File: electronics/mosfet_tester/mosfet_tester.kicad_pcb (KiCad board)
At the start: 2 copper layers, 25 parts, among them J101 BARREL_JACK, J102 CONN_01X06, J103 Screw_Terminal_1x01, J104 Screw_Terminal_1x01, J201 TEST_1P, J202 TEST_1P, J203 TEST_1P, J205 TEST_1P, J206 TEST_1P, J207 TEST_1P, Q201 Q_NMOS_GSD, U101 LM7805CT, U201 LM358

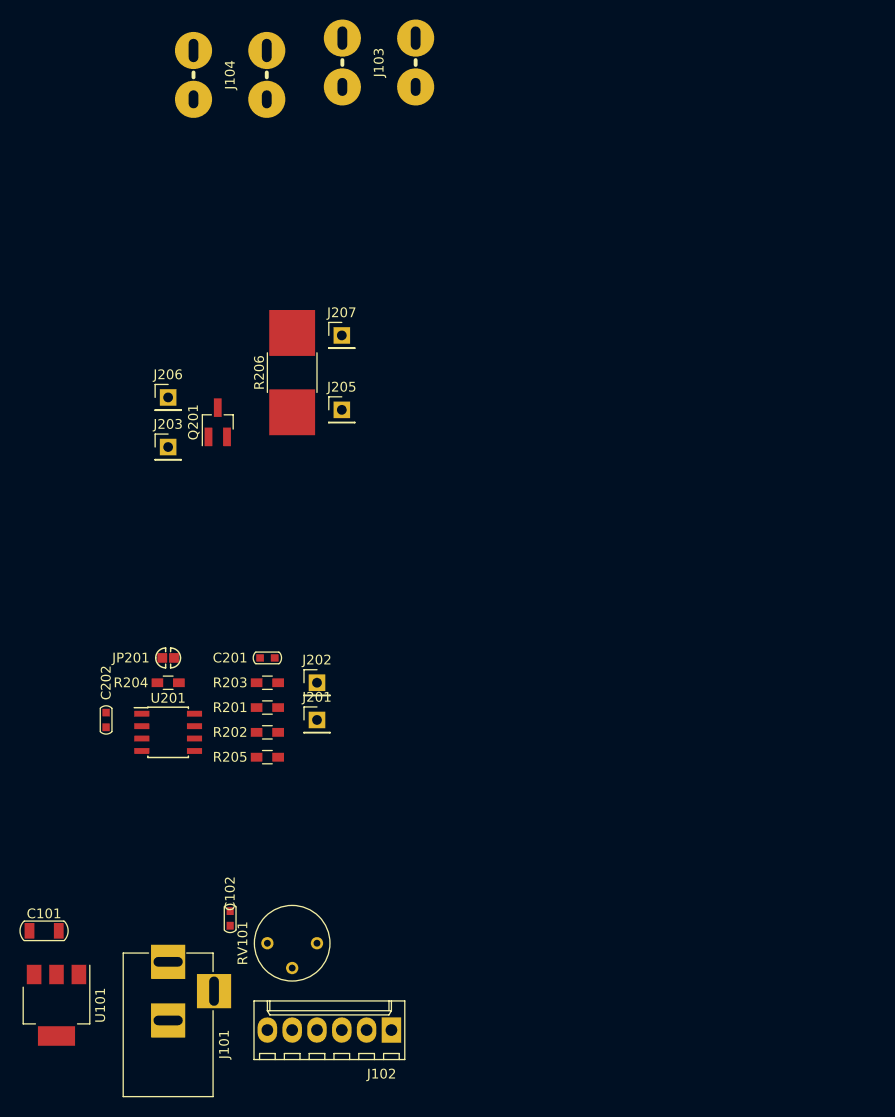
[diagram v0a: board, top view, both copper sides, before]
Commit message: Rework entire board, still in progress
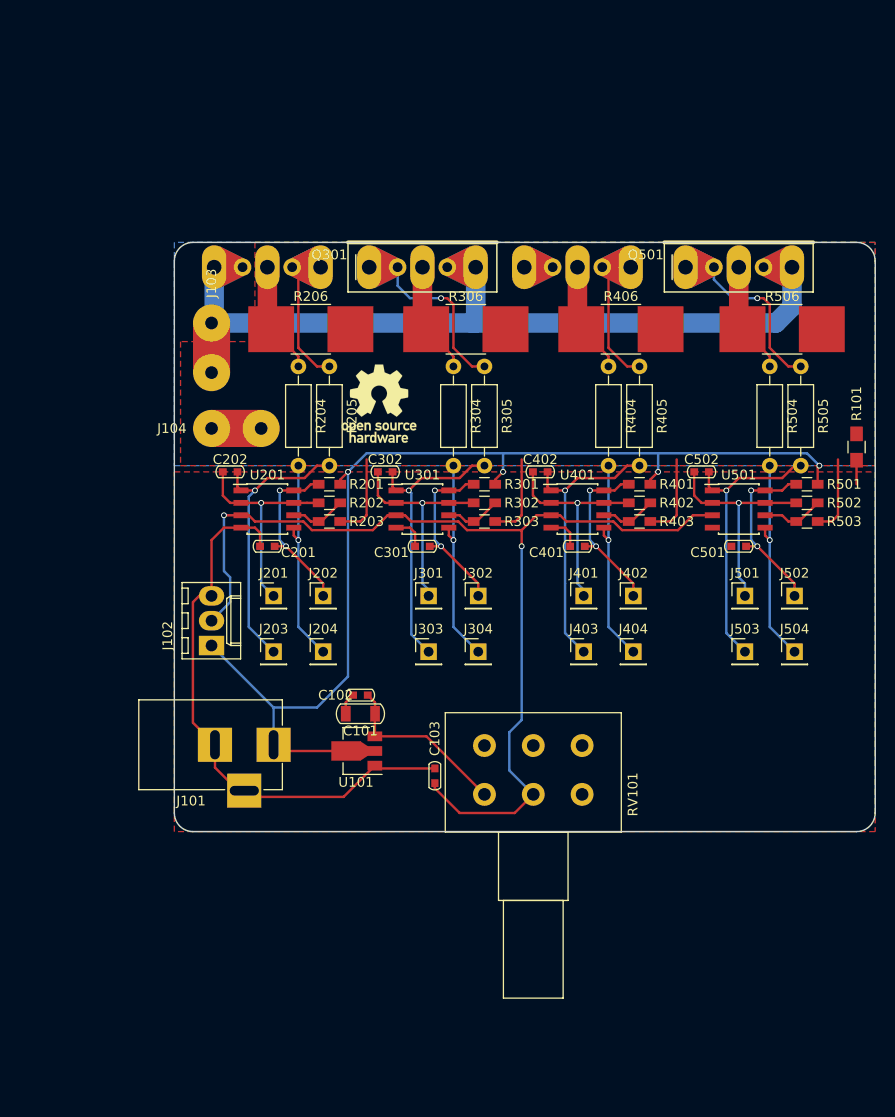
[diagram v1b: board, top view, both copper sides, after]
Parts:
- removed J206, J207: TEST_1P, Pin_Headers:Pin_Header_Straight_1x01_Pitch2.54mm
- removed JP201: Jumper_NC_Small, SolderJumpers:SJ_1_NO
- added C102: 0.1u, Capacitors_SMD_Round:C_0603, F.Cu at (135.3, 123.2)
- added C301: 0.1, Capacitors_SMD_Round:C_0603, F.Cu at (141.6, 108.0)
- added C302: C, Capacitors_SMD_Round:C_0603, F.Cu at (137.8, 100.3)
- added C401: 0.1, Capacitors_SMD_Round:C_0603, F.Cu at (157.5, 108.0)
- added C402: C, Capacitors_SMD_Round:C_0603, F.Cu at (153.7, 100.3)
- added C501: 0.1, Capacitors_SMD_Round:C_0603, F.Cu at (174.0, 108.0)
- added C502: C, Capacitors_SMD_Round:C_0603, F.Cu at (170.2, 100.3)
- added J301: TEST_1P, Pin_Headers:Pin_Header_Straight_1x01_Pitch2.54mm, F.Cu at (142.2, 113.0)
- added J302: TEST_1P, Pin_Headers:Pin_Header_Straight_1x01_Pitch2.54mm, F.Cu at (147.3, 113.0)
- added J303: TEST_1P, Pin_Headers:Pin_Header_Straight_1x01_Pitch2.54mm, F.Cu at (142.2, 118.7)
- added J304: TEST_1P, Pin_Headers:Pin_Header_Straight_1x01_Pitch2.54mm, F.Cu at (147.3, 118.7)
- added J401: TEST_1P, Pin_Headers:Pin_Header_Straight_1x01_Pitch2.54mm, F.Cu at (158.1, 113.0)
- added J402: TEST_1P, Pin_Headers:Pin_Header_Straight_1x01_Pitch2.54mm, F.Cu at (163.2, 113.0)
- added J403: TEST_1P, Pin_Headers:Pin_Header_Straight_1x01_Pitch2.54mm, F.Cu at (158.1, 118.7)
- added J404: TEST_1P, Pin_Headers:Pin_Header_Straight_1x01_Pitch2.54mm, F.Cu at (163.2, 118.7)
- added J501: TEST_1P, Pin_Headers:Pin_Header_Straight_1x01_Pitch2.54mm, F.Cu at (174.6, 113.0)
- added J502: TEST_1P, Pin_Headers:Pin_Header_Straight_1x01_Pitch2.54mm, F.Cu at (179.7, 113.0)
- added J503: TEST_1P, Pin_Headers:Pin_Header_Straight_1x01_Pitch2.54mm, F.Cu at (174.6, 118.7)
- added J504: TEST_1P, Pin_Headers:Pin_Header_Straight_1x01_Pitch2.54mm, F.Cu at (179.7, 118.7)
- added P101: OSHW, Symbols:OSHW-Logo_7.5x8mm_SilkScreen, F.Cu at (137.2, 93.3)
- added Q301: Q_NMOS_GSD, TO_Combo_Packages:TO_220_247, F.Cu at (141.6, 79.4)
- added Q401: Q_NMOS_GSD, TO_Combo_Packages:TO_220_247, B.Cu at (157.5, 79.4)
- added Q501: Q_NMOS_GSD, TO_Combo_Packages:TO_220_247, F.Cu at (174.0, 79.4)
- added R101: 0R, Resistors_SMD:R_0805_HandSoldering, F.Cu at (186.1, 97.8)
- added R301: 100R, Resistors_SMD:R_0603_HandSoldering, F.Cu at (148.0, 101.6)
- added R302: R, Resistors_SMD:R_0603_HandSoldering, F.Cu at (148.0, 103.5)
- added R303: R, Resistors_SMD:R_0603_HandSoldering, F.Cu at (148.0, 105.4)
- added R304: R, Resistors_THT:R_Axial_DIN0207_L6.3mm_D2.5mm_P10.16mm_Horizontal, F.Cu at (144.8, 89.5)
- added R305: R, Resistors_THT:R_Axial_DIN0207_L6.3mm_D2.5mm_P10.16mm_Horizontal, F.Cu at (148.0, 89.5)
- added R306: R, Resistors_SMD:R_2816_HandSoldering, F.Cu at (146.1, 85.7)
- added R401: 100R, Resistors_SMD:R_0603_HandSoldering, F.Cu at (163.8, 101.6)
- added R402: R, Resistors_SMD:R_0603_HandSoldering, F.Cu at (163.8, 103.5)
- added R403: R, Resistors_SMD:R_0603_HandSoldering, F.Cu at (163.8, 105.4)
- added R404: R, Resistors_THT:R_Axial_DIN0207_L6.3mm_D2.5mm_P10.16mm_Horizontal, F.Cu at (160.7, 89.5)
- added R405: R, Resistors_THT:R_Axial_DIN0207_L6.3mm_D2.5mm_P10.16mm_Horizontal, F.Cu at (163.8, 89.5)
- added R406: R, Resistors_SMD:R_2816_HandSoldering, F.Cu at (161.9, 85.7)
- added R501: 100R, Resistors_SMD:R_0603_HandSoldering, F.Cu at (181.0, 101.6)
- added R502: R, Resistors_SMD:R_0603_HandSoldering, F.Cu at (181.0, 103.5)
- added R503: R, Resistors_SMD:R_0603_HandSoldering, F.Cu at (181.0, 105.4)
- added R504: R, Resistors_THT:R_Axial_DIN0207_L6.3mm_D2.5mm_P10.16mm_Horizontal, F.Cu at (177.2, 89.5)
- added R505: R, Resistors_THT:R_Axial_DIN0207_L6.3mm_D2.5mm_P10.16mm_Horizontal, F.Cu at (180.3, 89.5)
- added R506: R, Resistors_SMD:R_2816_HandSoldering, F.Cu at (178.4, 85.7)
- added U301: LM358, Housings_SOIC:SOIC-8_3.9x4.9mm_Pitch1.27mm, F.Cu at (141.6, 104.1)
- added U401: LM358, Housings_SOIC:SOIC-8_3.9x4.9mm_Pitch1.27mm, F.Cu at (157.5, 104.1)
- added U501: LM358, Housings_SOIC:SOIC-8_3.9x4.9mm_Pitch1.27mm, F.Cu at (174.0, 104.1)
- C101: value C -> 22u
- J102: value CONN_01X06 -> CONN_01X03; footprint Connectors_Molex:Molex_KK-6410-06_06x2.54mm_Straight -> Connectors_Molex:Molex_KK-6410-03_03x2.54mm_Straight
- J103, J104: footprint Screw_Connectors:4_Pin_Screw_Connector -> Screw_Connectors:2_Pin_Quick_Fit
- Q201: footprint TO_SOT_Packages_SMD:SOT-23_Handsoldering -> TO_Combo_Packages:TO_220_247; moved to B.Cu
- R204, R205: footprint Resistors_SMD:R_0603_HandSoldering -> Resistors_THT:R_Axial_DIN0207_L6.3mm_D2.5mm_P10.16mm_Horizontal
- RV101: footprint Potentiometers:Potentiometer_Trimmer_Bourns_3339P_Horizontal -> Potentiometers:Potentiometer_Alps_RK163_Double_Vertical
- U101: value LM7805CT -> MCP1703A-3302/MB; footprint TO_SOT_Packages_SMD:SOT-223-3Lead_TabPin2 -> TO_SOT_Packages_SMD:SOT89-3_Housing
- moved J102 43.5 mm to (120.0, 118.1), turned to 90 degrees
- moved U101 40.6 mm to (135.3, 128.9), turned to 180 degrees
- moved R205 40.5 mm to (132.1, 89.5), turned to 270 degrees
- moved C101 39.3 mm to (135.3, 125.1), turned to 180 degrees
- moved J104 36.2 mm to (122.6, 95.9), turned to 0 degrees
- moved R204 35.0 mm to (128.9, 89.5), turned to 270 degrees
- moved J103 33.9 mm to (120.0, 87.6), turned to 270 degrees
- moved C202 28.4 mm to (121.9, 100.3), turned to 180 degrees
- moved C103 25.5 mm to (142.9, 131.4)
- moved U201 25.0 mm to (125.7, 104.1)
- moved J204 24.8 mm to (131.4, 118.7)
- moved J101 24.7 mm to (126.4, 128.3), turned to 0 degrees
- moved R202 24.3 mm to (132.1, 103.5)
- moved R201 23.7 mm to (132.1, 101.6)
- moved J203 23.6 mm to (126.4, 118.7)
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- renumbered C102 to C103, J205 to J204
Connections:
- C103 pad 1: /slice/5V_REF -> /slice1/5V_REF
- C202 pad 1: Net-(C202-Pad1) -> /slice1/Vgs
- J102 pad 1: /slice/Vgs -> +12V
- J102 pad 2: (no net) -> /slice1/5V_REF
- J102 pad 3: (no net) -> GND
- J103 pad 1: GND -> /slice1/VIN+
- J104 pad 1: /slice/VIN+ -> /slice1/VIN-
- J203 pad 1: /slice/Vgs -> /slice1/Vgs
- J204 pad 1: Net-(J205-Pad1) -> Net-(J204-Pad1)
- Q201 pad 1: /slice/Vgs -> Net-(Q201-Pad1)
- Q201 pad 2: Net-(J205-Pad1) -> Net-(Q201-Pad2)
- Q201 pad 3: /slice/VIN+ -> /slice1/VIN+
- R203 pad 1: Net-(JP201-Pad1) -> /slice1/VIN-
- R204 pad 1: /slice/Vgs -> Net-(Q201-Pad2)
- R204 pad 2: Net-(C202-Pad1) -> Net-(J204-Pad1)
- R205 pad 1: Net-(J205-Pad1) -> Net-(Q201-Pad1)
- R205 pad 2: Net-(R205-Pad2) -> /slice1/Vgs
- R206 pad 1: Net-(J205-Pad1) -> Net-(Q201-Pad2)
- R206 pad 2: GND -> /slice1/VIN-
- RV101 pad 2: /slice/5V_REF -> /slice1/5V_REF
- U101 pad 1: +12V -> GND
- U101 pad 2: GND -> +12V
- U201 pad 1: Net-(C202-Pad1) -> /slice1/Vgs
- U201 pad 3: /slice/5V_REF -> /slice1/5V_REF
- U201 pad 5: Net-(R205-Pad2) -> Net-(J204-Pad1)
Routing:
- net +12V: track 0.00 -> 111.5 mm, vias 0 -> 4
- net /slice1/5V_REF: track 0.00 -> 106.8 mm, vias 0 -> 2
- net /slice1/VIN+: track 0.00 -> 96.7 mm
- net GND: track 0.00 -> 69.2 mm
- net /slice1/VIN-: track 0.00 -> 34.1 mm
- net /slice1/Vgs: track 0.00 -> 30.0 mm, vias 0 -> 1
- net /slice2/Vgs: track 0.00 -> 29.5 mm, vias 0 -> 1
- net /slice3/Vgs: track 0.00 -> 29.5 mm, vias 0 -> 1
- net /slice4/Vgs: track 0.00 -> 29.5 mm, vias 0 -> 1
- net Net-(C502-Pad2): track 0.00 -> 23.0 mm, vias 0 -> 1
- net Net-(J404-Pad1): track 0.00 -> 22.9 mm, vias 0 -> 1
- net Net-(J204-Pad1): track 0.00 -> 22.9 mm, vias 0 -> 1
- net Net-(C202-Pad2): track 0.00 -> 22.6 mm, vias 0 -> 1
- net Net-(C402-Pad2): track 0.00 -> 22.3 mm, vias 0 -> 1
- net Net-(C302-Pad2): track 0.00 -> 22.3 mm, vias 0 -> 1
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- added copper zone on B.Cu, net /slice1/VIN+
- added copper zone on F.Cu, net /slice1/VIN-
- added copper zone on F.Cu, net GND
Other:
- board outline added: 71.8 x 60.3 mm
